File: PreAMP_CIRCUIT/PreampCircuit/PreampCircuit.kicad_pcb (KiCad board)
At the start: 2 copper layers, 41 x 35.5 mm, 10 parts, among them J2 Conn_01x02_Pin, Q2 2N3819

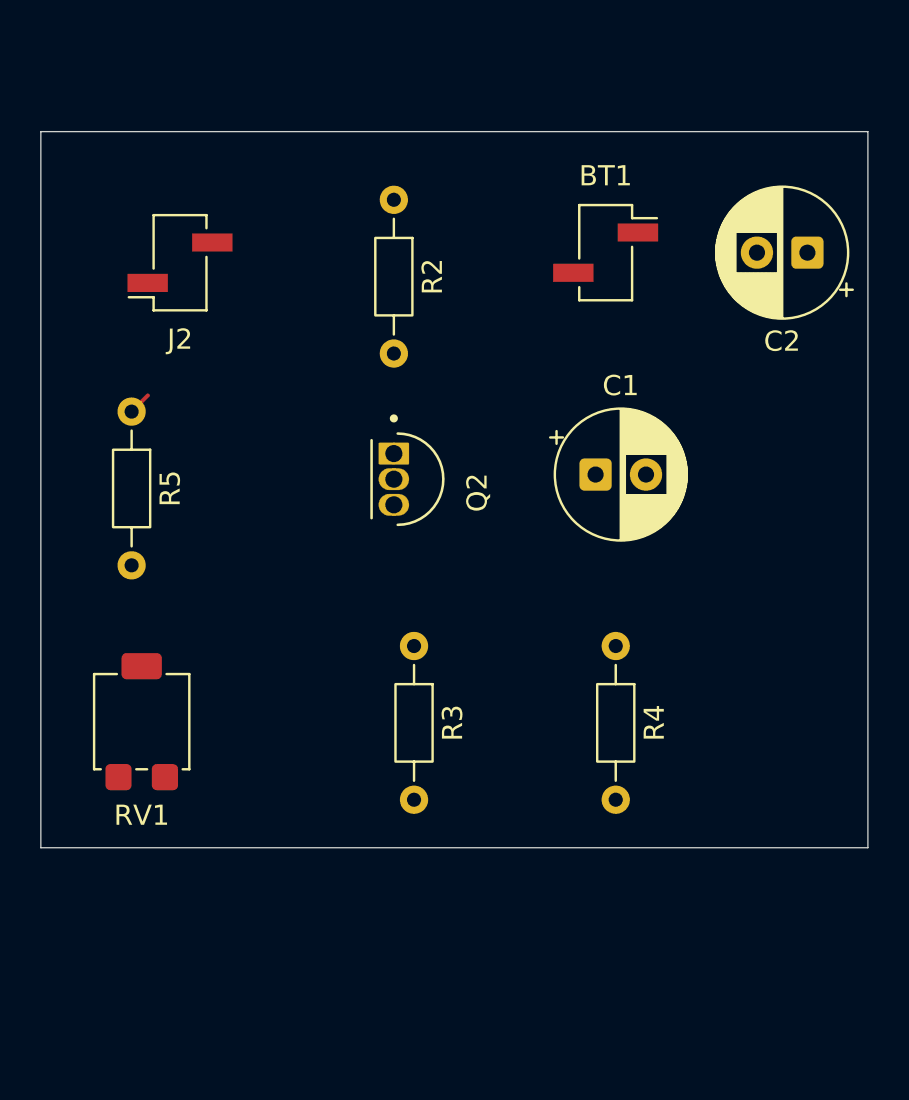
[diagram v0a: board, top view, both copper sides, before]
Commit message: ROUTING
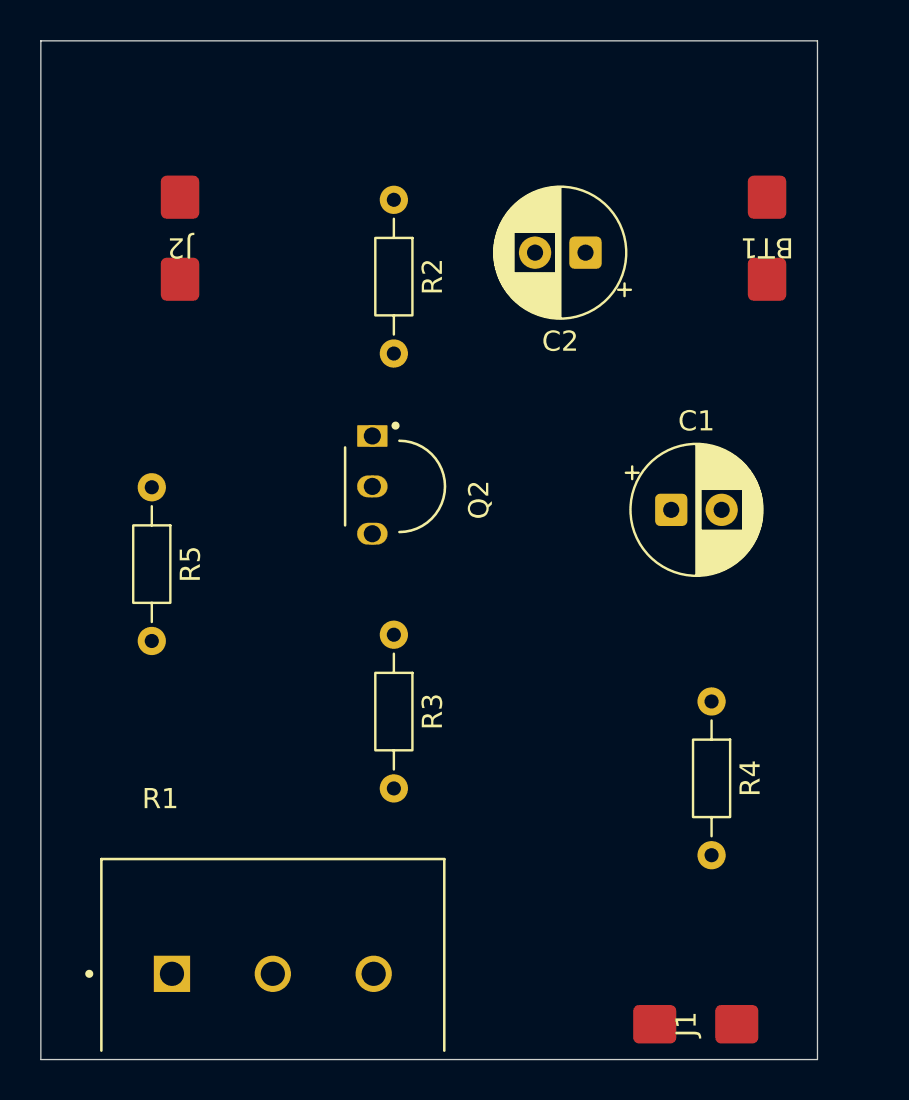
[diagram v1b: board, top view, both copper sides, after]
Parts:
- removed RV1: R_Pot 3M, Potentiometer_SMD:Potentiometer_Bourns_3314G_Vertical
- added J1: AudioJack2, 2pads:2pads, F.Cu at (124.0, 80.8)
- added R1: PTN16-A10220K1B1, pot:POT_PTN16-A10220K1B1, F.Cu at (98.0, 78.2)
- BT1, J2: footprint Connector_PinSocket_2.00mm:PinSocket_1x02_P2.00mm_Vertical_SMD_Pin1Right -> 2pads:2pads
- moved C2 11.0 mm to (118.5, 42.5)
- moved BT1 8.04 mm to (127.5, 41.8), turned to 180 degrees
- moved R4 5.49 mm to (124.8, 64.8)
- moved C1 4.14 mm to (122.8, 55.2)
- moved R5 3.88 mm to (97.0, 54.1)
- moved J2 1.25 mm to (98.4, 41.8)
- moved R3 1.15 mm to (109.0, 61.4)
- moved Q2 0.37 mm to (109.1, 54.1)
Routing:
- net Net-(J2-Pin_1): track 1.13 -> 0.00 mm
- net Net-(R1-Pad2): track 0.71 -> 0.00 mm
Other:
- board size 41 x 35.5 mm -> 38.5 x 50.5 mm
